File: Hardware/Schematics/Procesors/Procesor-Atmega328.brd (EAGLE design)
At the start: 27.3 x 27.3 mm, 6 parts

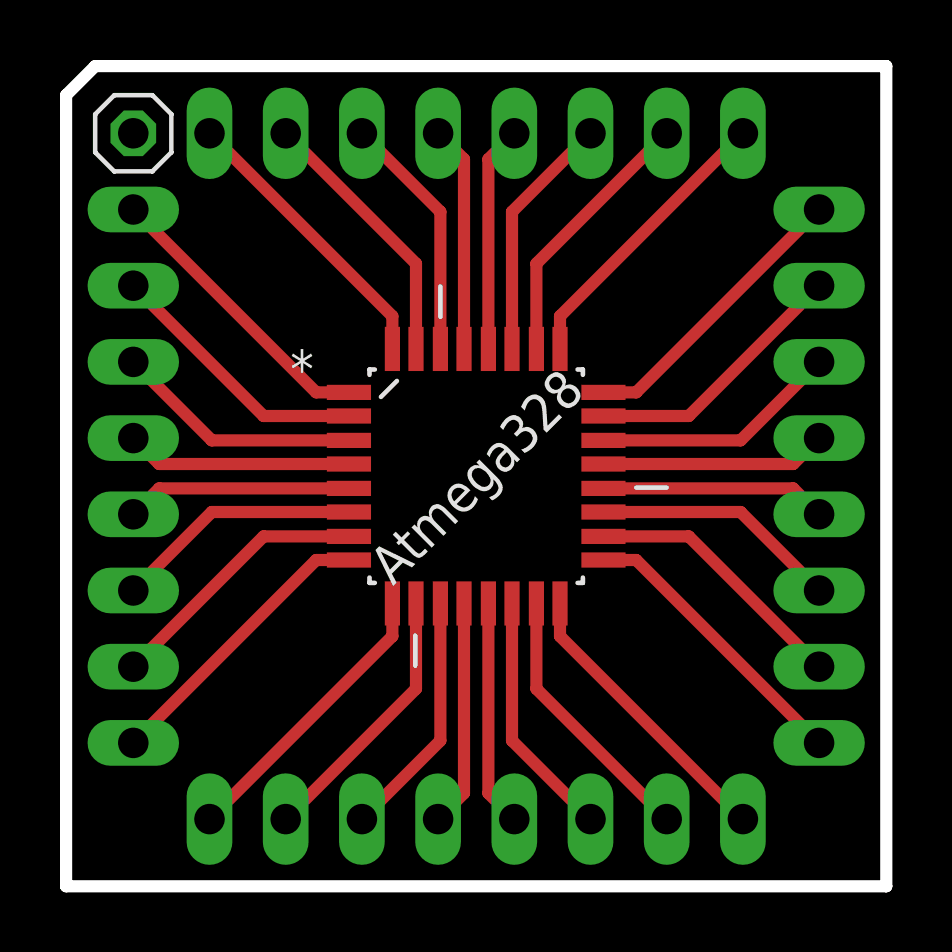
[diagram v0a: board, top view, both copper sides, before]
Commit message: 3D package upgrade
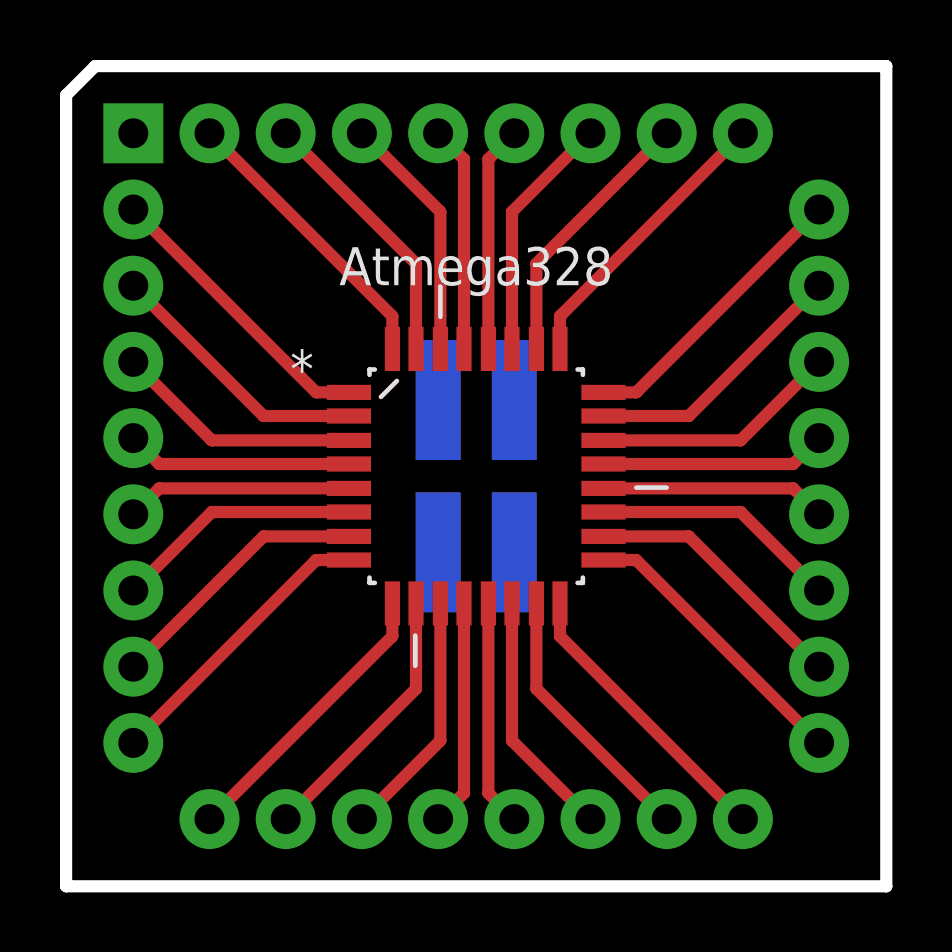
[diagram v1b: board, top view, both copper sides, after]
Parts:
- removed E$1: (no value), pinhead:1X01
- removed E$10, E$11, E$12, E$9: (no value), pinhead:1X08
- added E$2: (no value), Cing Library:PROCESSOR-SOCKET_PCB
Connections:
- net S$1: now also E$2.D2; no longer E$10.8
- net S$10: now also E$2.A0; no longer E$11.2
- net S$11: now also E$2.A7; no longer E$11.3
- net S$12: now also E$2.GND3; no longer E$11.4
- net S$13: now also E$2.AREF; no longer E$11.5
- net S$14: now also E$2.A6; no longer E$11.6
- net S$15: now also E$2.VCC3; no longer E$11.7
- net S$16: now also E$2.D13; no longer E$11.8
- net S$17: now also E$2.D12; no longer E$12.8
- net S$18: now also E$2.D11; no longer E$12.7
- net S$19: now also E$2.D10; no longer E$12.6
- net S$2: now also E$2.D1; no longer E$10.7
- net S$20: now also E$2.D9; no longer E$12.5
- net S$21: now also E$2.D8; no longer E$12.4
- net S$22: now also E$2.D7; no longer E$12.3
- net S$23: now also E$2.D6; no longer E$12.2
- net S$24: now also E$2.D5; no longer E$12.1
- net S$25: now also E$2.CRYST2; no longer E$9.1
- net S$26: now also E$2.CRYST1; no longer E$9.2
- net S$27: now also E$2.VCC2; no longer E$9.3
- net S$28: now also E$2.GND2; no longer E$9.4
- net S$29: now also E$2.VCC; no longer E$9.5
- net S$3: now also E$2.D0; no longer E$10.6
- net S$30: now also E$2.GND; no longer E$9.6
- net S$31: now also E$2.D4; no longer E$9.7
- net S$32: now also E$2.D3; no longer E$9.8
- net S$4: now also E$2.RESET; no longer E$10.5
- net S$5: now also E$2.A5; no longer E$10.4
- net S$6: now also E$2.A4; no longer E$10.3
- net S$7: now also E$2.A3; no longer E$10.2
- net S$8: now also E$2.A2; no longer E$10.1
- net S$9: now also E$2.A1; no longer E$11.1
